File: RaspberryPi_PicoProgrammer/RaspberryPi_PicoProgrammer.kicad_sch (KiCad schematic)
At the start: 7 parts, among them J1 Conn_02x05_Odd_Even, J2 Conn_01x03_Male, J3 Conn_02x03_Odd_Even, J4 BM03B-SRSS-TBLFSN, J5 Raspberry_Pi_2_3

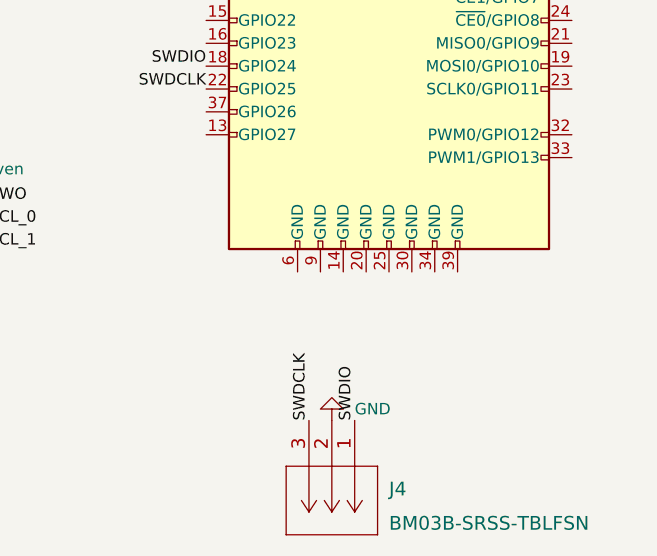
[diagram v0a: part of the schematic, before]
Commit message: board sent out
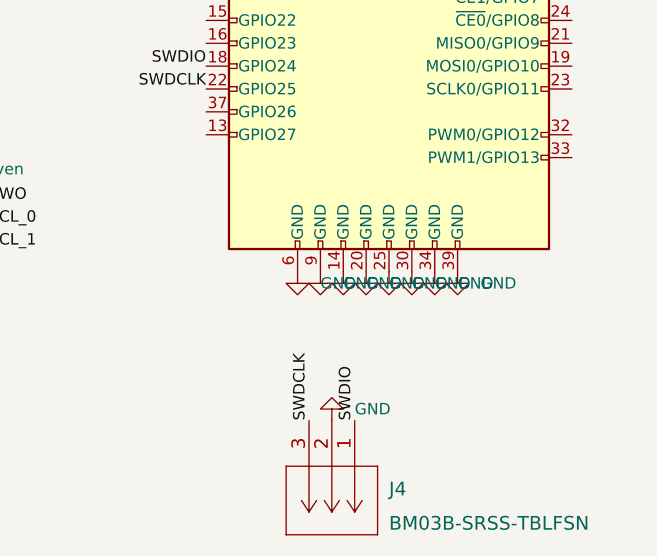
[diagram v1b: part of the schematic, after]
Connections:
- net GND: now also J5.14 (GND), J5.20 (GND), J5.25 (GND), J5.30 (GND), J5.34 (GND), J5.39 (GND), J5.6 (GND), J5.9 (GND)
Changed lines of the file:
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@@
     (pin "2")
+  )
+  (symbol (lib_id "power:GND") (at 172.72 109.22 0) (unit 1)
+    (in_bom yes) (on_board yes) (fields_autoplaced)
+    (property "Reference" "#PWR?" (id 0) (at 172.72 115.57 0)
+      (effects (font (size 1.27 1.27)) hide)
+    )
+    (property "Value" "GND" (id 1) (at 175.26 110.4899 0)
+      (effects (font (size 1.27 1.27)) (justify left))
+    )
+    (property "Footprint" "" (id 2) (at 172.72 109.22 0)
+      (effects (font (size 1.27 1.27)) hide)
+    )
+    (property "Datasheet" "" (id 3) (at 172.72 109.22 0)
+      (effects (font (size 1.27 1.27)) hide)
+    )
+    (pin "1")
   )
   (symbol (lib_id "Connector:Raspberry_Pi_2_3") (at 175.26 76.2 0) (unit 1)
@@
     (pin "2")
   )
+  (symbol (lib_id "power:GND") (at 182.88 109.22 0) (unit 1)
+    (in_bom yes) (on_board yes) (fields_autoplaced)
+    (property "Reference" "#PWR?" (id 0) (at 182.88 115.57 0)
+      (effects (font (size 1.27 1.27)) hide)
+    )
+    (property "Value" "GND" (id 1) (at 185.42 110.4899 0)
+      (effects (font (size 1.27 1.27)) (justify left))
+    )
+    (property "Footprint" "" (id 2) (at 182.88 109.22 0)
+      (effects (font (size 1.27 1.27)) hide)
+    )
+    (property "Datasheet" "" (id 3) (at 182.88 109.22 0)
+      (effects (font (size 1.27 1.27)) hide)
+    )
+    (pin "1")
+  )
+  (symbol (lib_id "power:GND") (at 175.26 109.22 0) (unit 1)
+    (in_bom yes) (on_board yes) (fields_autoplaced)
+    (property "Reference" "#PWR?" (id 0) (at 175.26 115.57 0)
+      (effects (font (size 1.27 1.27)) hide)
+    )
+    (property "Value" "GND" (id 1) (at 177.8 110.4899 0)
+      (effects (font (size 1.27 1.27)) (justify left))
+    )
+    (property "Footprint" "" (id 2) (at 175.26 109.22 0)
+      (effects (font (size 1.27 1.27)) hide)
+    )
+    (property "Datasheet" "" (id 3) (at 175.26 109.22 0)
+      (effects (font (size 1.27 1.27)) hide)
+    )
+    (pin "1")
+  )
   (symbol (lib_id "Connector:Conn_01x03_Male") (at 121.92 36.83 0) (unit 1)
     (in_bom yes) (on_board yes) (fields_autoplaced)
@@
     (pin "9")
   )
+  (symbol (lib_id "power:GND") (at 167.64 109.22 0) (unit 1)
+    (in_bom yes) (on_board yes) (fields_autoplaced)
+    (property "Reference" "#PWR?" (id 0) (at 167.64 115.57 0)
+      (effects (font (size 1.27 1.27)) hide)
+    )
+    (property "Value" "GND" (id 1) (at 170.18 110.4899 0)
+      (effects (font (size 1.27 1.27)) (justify left))
+    )
+    (property "Footprint" "" (id 2) (at 167.64 109.22 0)
+      (effects (font (size 1.27 1.27)) hide)
+    )
+    (property "Datasheet" "" (id 3) (at 167.64 109.22 0)
+      (effects (font (size 1.27 1.27)) hide)
+    )
+    (pin "1")
+  )
+  (symbol (lib_id "power:GND") (at 165.1 109.22 0) (unit 1)
+    (in_bom yes) (on_board yes) (fields_autoplaced)
+    (property "Reference" "#PWR?" (id 0) (at 165.1 115.57 0)
+      (effects (font (size 1.27 1.27)) hide)
+    )
+    (property "Value" "GND" (id 1) (at 167.64 110.4899 0)
+      (effects (font (size 1.27 1.27)) (justify left))
+    )
+    (property "Footprint" "" (id 2) (at 165.1 109.22 0)
+      (effects (font (size 1.27 1.27)) hide)
+    )
+    (property "Datasheet" "" (id 3) (at 165.1 109.22 0)
+      (effects (font (size 1.27 1.27)) hide)
+    )
+    (pin "1")
+  )
+  (symbol (lib_id "power:GND") (at 177.8 109.22 0) (unit 1)
+    (in_bom yes) (on_board yes) (fields_autoplaced)
+    (property "Reference" "#PWR?" (id 0) (at 177.8 115.57 0)
+      (effects (font (size 1.27 1.27)) hide)
+    )
+    (property "Value" "GND" (id 1) (at 180.34 110.4899 0)
+      (effects (font (size 1.27 1.27)) (justify left))
+    )
+    (property "Footprint" "" (id 2) (at 177.8 109.22 0)
+      (effects (font (size 1.27 1.27)) hide)
+    )
+    (property "Datasheet" "" (id 3) (at 177.8 109.22 0)
+      (effects (font (size 1.27 1.27)) hide)
+    )
+    (pin "1")
+  )
+  (symbol (lib_id "power:GND") (at 180.34 109.22 0) (unit 1)
+    (in_bom yes) (on_board yes) (fields_autoplaced)
+    (property "Reference" "#PWR?" (id 0) (at 180.34 115.57 0)
+      (effects (font (size 1.27 1.27)) hide)
+    )
+    (property "Value" "GND" (id 1) (at 182.88 110.4899 0)
+      (effects (font (size 1.27 1.27)) (justify left))
+    )
+    (property "Footprint" "" (id 2) (at 180.34 109.22 0)
+      (effects (font (size 1.27 1.27)) hide)
+    )
+    (property "Datasheet" "" (id 3) (at 180.34 109.22 0)
+      (effects (font (size 1.27 1.27)) hide)
+    )
+    (pin "1")
+  )
   (symbol (lib_id "Connector_Generic:Conn_02x03_Odd_Even") (at 123.19 104.14 0) (unit 1)
     (in_bom yes) (on_board yes) (fields_autoplaced)
@@
     (pin "3")
   )
+  (symbol (lib_id "power:GND") (at 170.18 109.22 0) (unit 1)
+    (in_bom yes) (on_board yes) (fields_autoplaced)
+    (property "Reference" "#PWR?" (id 0) (at 170.18 115.57 0)
+      (effects (font (size 1.27 1.27)) hide)
+    )
+    (property "Value" "GND" (id 1) (at 172.72 110.4899 0)
+      (effects (font (size 1.27 1.27)) (justify left))
+    )
+    (property "Footprint" "" (id 2) (at 170.18 109.22 0)
+      (effects (font (size 1.27 1.27)) hide)
+    )
+    (property "Datasheet" "" (id 3) (at 170.18 109.22 0)
+      (effects (font (size 1.27 1.27)) hide)
+    )
+    (pin "1")
+  )
   (symbol (lib_id "power:GND") (at 102.87 66.04 270) (unit 1)
     (in_bom yes) (on_board yes) (fields_autoplaced)
@@
       (reference "#PWR0103") (unit 1) (value "GND") (footprint "")
     )
+    (path "/148c1fef-b661-460b-a57a-325322a15ece"
+      (reference "#PWR?") (unit 1) (value "GND") (footprint "")
+    )
     (path "/2dc3733a-9d58-4877-8e6e-e1d8cbfa0c4a"
       (reference "#PWR?") (unit 1) (value "GND") (footprint "")
     )
+    (path "/3146ca1f-eed7-4baa-9733-67c1d02e5784"
+      (reference "#PWR?") (unit 1) (value "GND") (footprint "")
+    )
+    (path "/60940c6c-27ab-4fda-8fce-85de9b7166e0"
+      (reference "#PWR?") (unit 1) (value "GND") (footprint "")
+    )
+    (path "/ab3158bc-e462-4ae6-93b7-eb9a1d8fd8be"
+      (reference "#PWR?") (unit 1) (value "GND") (footprint "")
+    )
+    (path "/af81e9b3-8f66-48b0-834e-d6d8bce921bf"
+      (reference "#PWR?") (unit 1) (value "GND") (footprint "")
+    )
+    (path "/b24511b1-2c84-43ba-8736-fb8e70ff6c1d"
+      (reference "#PWR?") (unit 1) (value "GND") (footprint "")
+    )
+    (path "/cd4f74bf-5bbd-453d-bf71-0d8a83165477"
+      (reference "#PWR?") (unit 1) (value "GND") (footprint "")
+    )
+    (path "/fddcbc36-8d82-4d5d-9795-3829c0452e89"
+      (reference "#PWR?") (unit 1) (value "GND") (footprint "")
+    )
